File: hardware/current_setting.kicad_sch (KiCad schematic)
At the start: 10 parts, among them U2 ADTL084

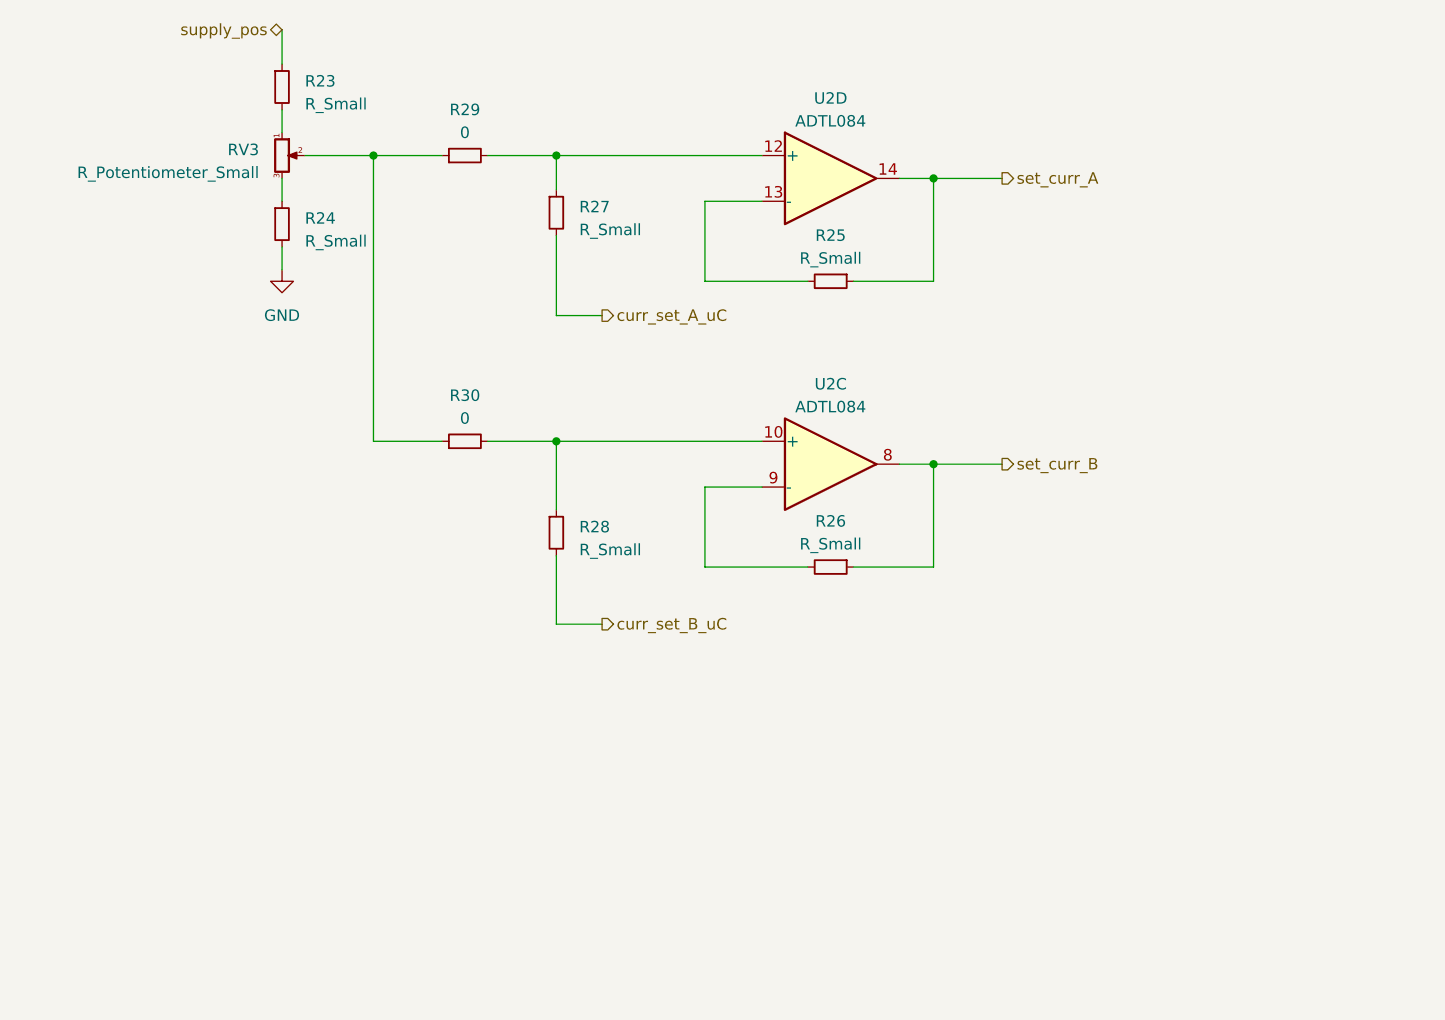
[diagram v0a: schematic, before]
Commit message: Updates to structure of the schematic. Minor funcitonality adjustments.
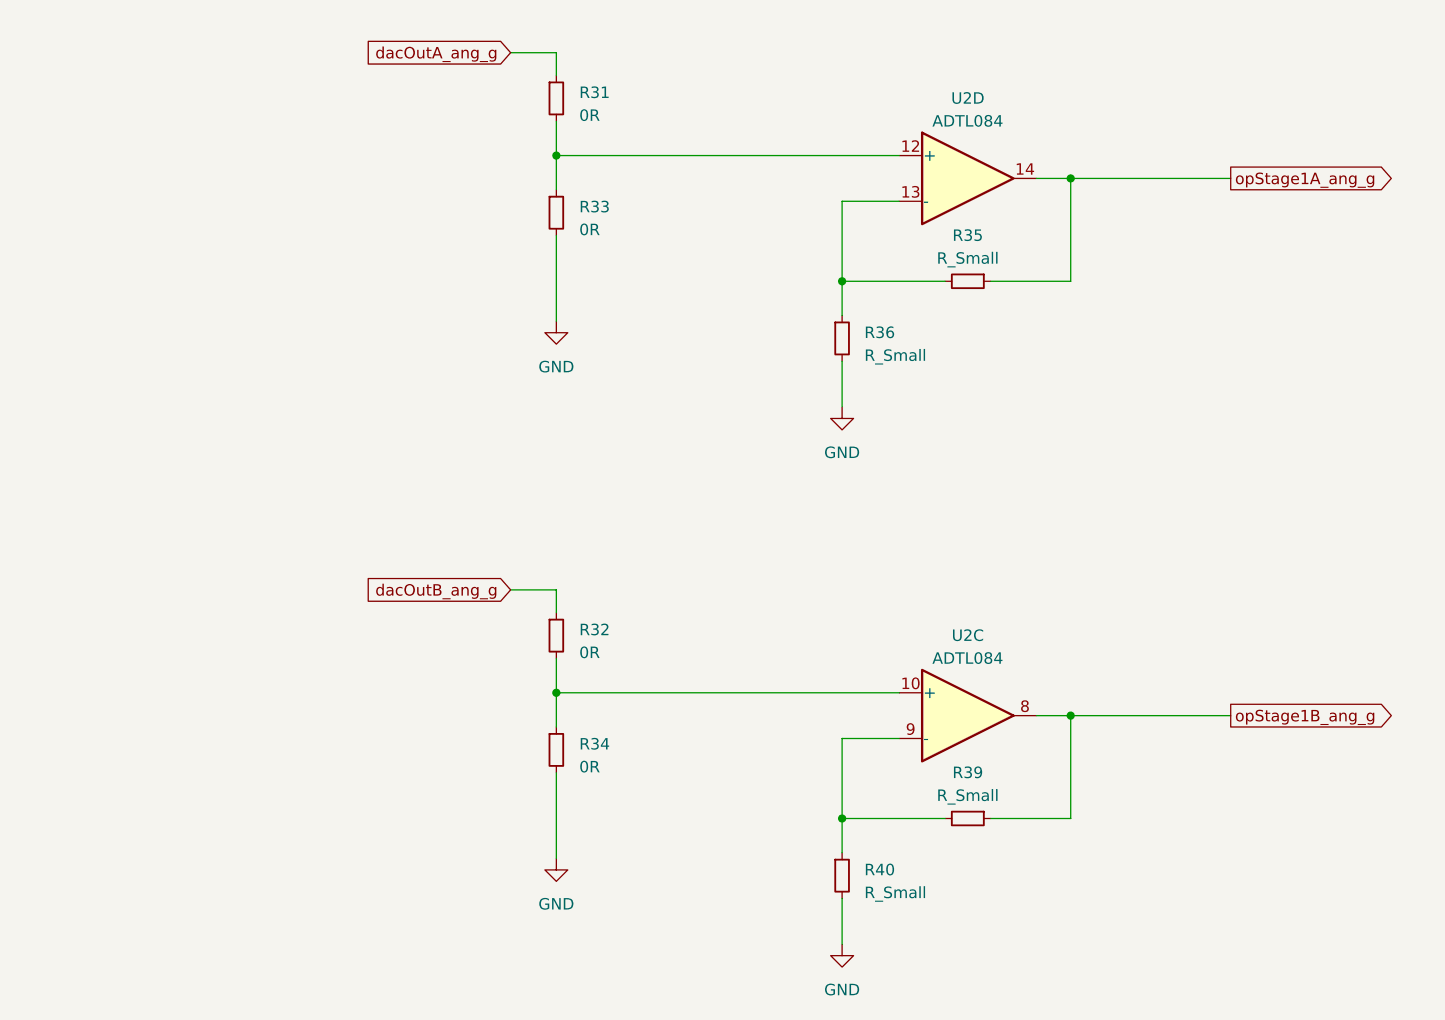
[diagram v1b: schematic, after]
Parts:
- removed R23, R24, R28: R_Small, symbol Device:R_Small
- removed R29, R30: 0, symbol Device:R_Small
- removed RV3: R_Potentiometer_Small, symbol Device:R_Potentiometer_Small
- added R31, R32, R34: 0R, Resistor_SMD:R_0805_2012Metric_Pad1.20x1.40mm_HandSolder, symbol Device:R_Small
- added R36, R40: R_Small, Resistor_SMD:R_0805_2012Metric_Pad1.20x1.40mm_HandSolder, symbol Device:R_Small
- R33: renamed from R27; value R_Small -> 0R; footprint (none) -> Resistor_SMD:R_0805_2012Metric_Pad1.20x1.40mm_HandSolder
- R35: renamed from R25; footprint (none) -> Resistor_SMD:R_0805_2012Metric_Pad1.20x1.40mm_HandSolder
- R39: renamed from R26; footprint (none) -> Resistor_SMD:R_0805_2012Metric_Pad1.20x1.40mm_HandSolder
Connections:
- net curr_set_A_uC is gone; now on net GND: R33.2
- net GND: now also R34.2, R36.2, R40.2
- net at R33.1, U2.12 (+): now also R31.2
- net at U2.10 (+): now also R32.2, R34.1
- net at R35.2, U2.13 (-): now also R36.1
- net at R39.2, U2.9 (-): now also R40.1
- net set_curr_A renamed opStage1A_ang_g
- net set_curr_B renamed opStage1B_ang_g
- new net dacOutA_ang_g: R31.1
- new net dacOutB_ang_g: R32.1
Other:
- moved on the sheet: R35, R39, U2C, U2D
